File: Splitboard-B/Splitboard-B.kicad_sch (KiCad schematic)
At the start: 133 parts, among them J1 USB_C_Receptacle, J2 Conn_01x09, K1 KEYSW, K10 KEYSW, K11 KEYSW, K12 KEYSW, K13 KEYSW, K14 KEYSW, K15 KEYSW, K16 KEYSW, K17 KEYSW, K18 KEYSW, K19 KEYSW, K2 KEYSW, K20 KEYSW, K21 KEYSW, K22 KEYSW, K23 KEYSW, K24 KEYSW, K25 KEYSW, K26 KEYSW, K27 KEYSW, K28 KEYSW, K29 KEYSW, K3 KEYSW, K30 KEYSW, K31 KEYSW, K32 KEYSW, K33 KEYSW, K34 KEYSW, K35 KEYSW, K36 KEYSW, K37 KEYSW, K38 KEYSW, K4 KEYSW, K5 KEYSW, K6 KEYSW, K7 KEYSW, K8 KEYSW, K9 KEYSW, SW1 RotaryEncoder, U1 CR2013-MI2120, U2 MCP23017_SP, U3 AMS1117-3.3

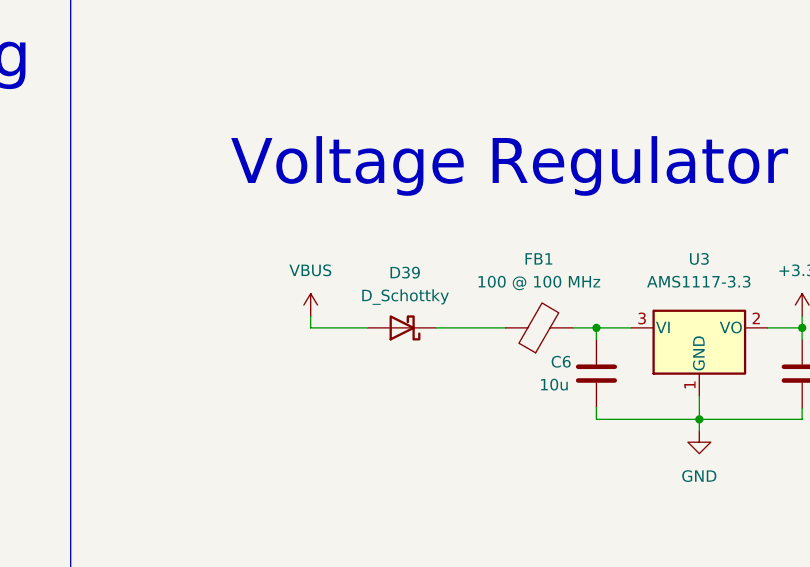
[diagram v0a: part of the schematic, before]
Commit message: Layout changes
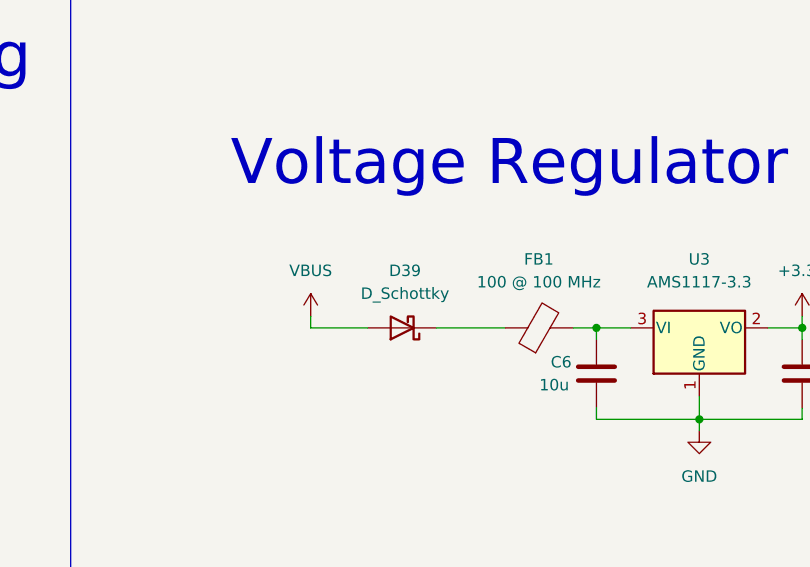
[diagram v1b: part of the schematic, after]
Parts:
- D39: footprint Diode_SMD:D_SOD-123 -> Diode_SMD:D_SOD-323
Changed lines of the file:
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@@
   (symbol (lib_id "Device:D_Schottky") (at 222.25 233.68 180) (unit 1)
     (in_bom yes) (on_board yes) (fields_autoplaced)
-    (property "Reference" "D39" (id 0) (at 222.5675 227.584 0))
-    (property "Value" "D_Schottky" (id 1) (at 222.5675 230.124 0))
-    (property "Footprint" "Diode_SMD:D_SOD-123" (id 2) (at 222.25 233.68 0)
+    (property "Reference" "D39" (id 0) (at 222.5675 227.33 0))
+    (property "Value" "D_Schottky" (id 1) (at 222.5675 229.87 0))
+    (property "Footprint" "Diode_SMD:D_SOD-323" (id 2) (at 222.25 233.68 0)
       (effects (font (size 1.27 1.27)) hide)
     )
@@
     )
     (path "/eb775797-25c2-4116-bc6c-2239b2291c1a"
-      (reference "D39") (unit 1) (value "D_Schottky") (footprint "Diode_SMD:D_SOD-123")
+      (reference "D39") (unit 1) (value "D_Schottky") (footprint "Diode_SMD:D_SOD-323")
     )
     (path "/f5b7f673-4d4e-4451-93c3-b001e2dc606f"
